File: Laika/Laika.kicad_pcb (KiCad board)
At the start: 2 copper layers, 70 x 70 mm, 29 parts, among them J1 A-DF_09_A_KG-T4S, J2 Micro_SD_Card, J3 0436500300, U1 LSM6DSL, U2 MS5611-01BA, U3 RASPBERRY_PI_ZERO_2_W, U4 MMC5983MA, U5 H3LIS331DLTR, U6 THVD1451D

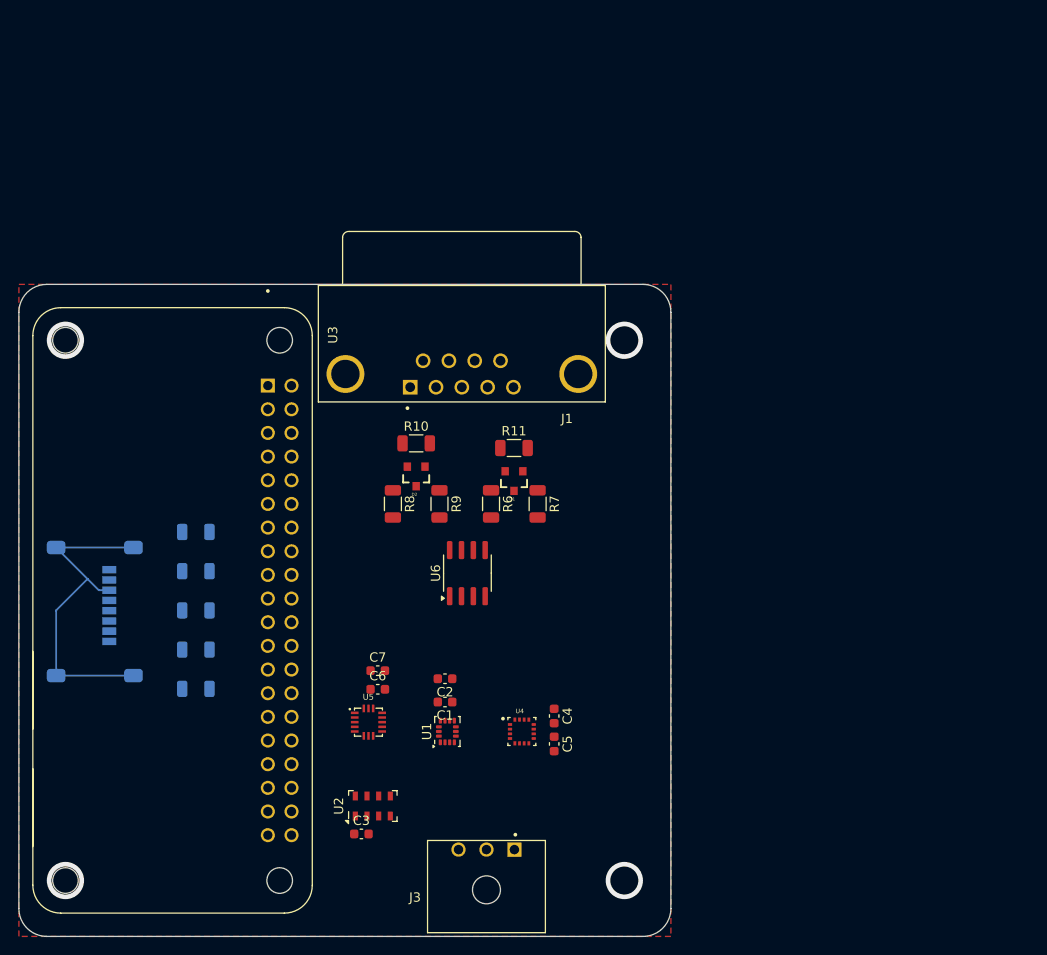
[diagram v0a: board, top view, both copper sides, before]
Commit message: Version 0A
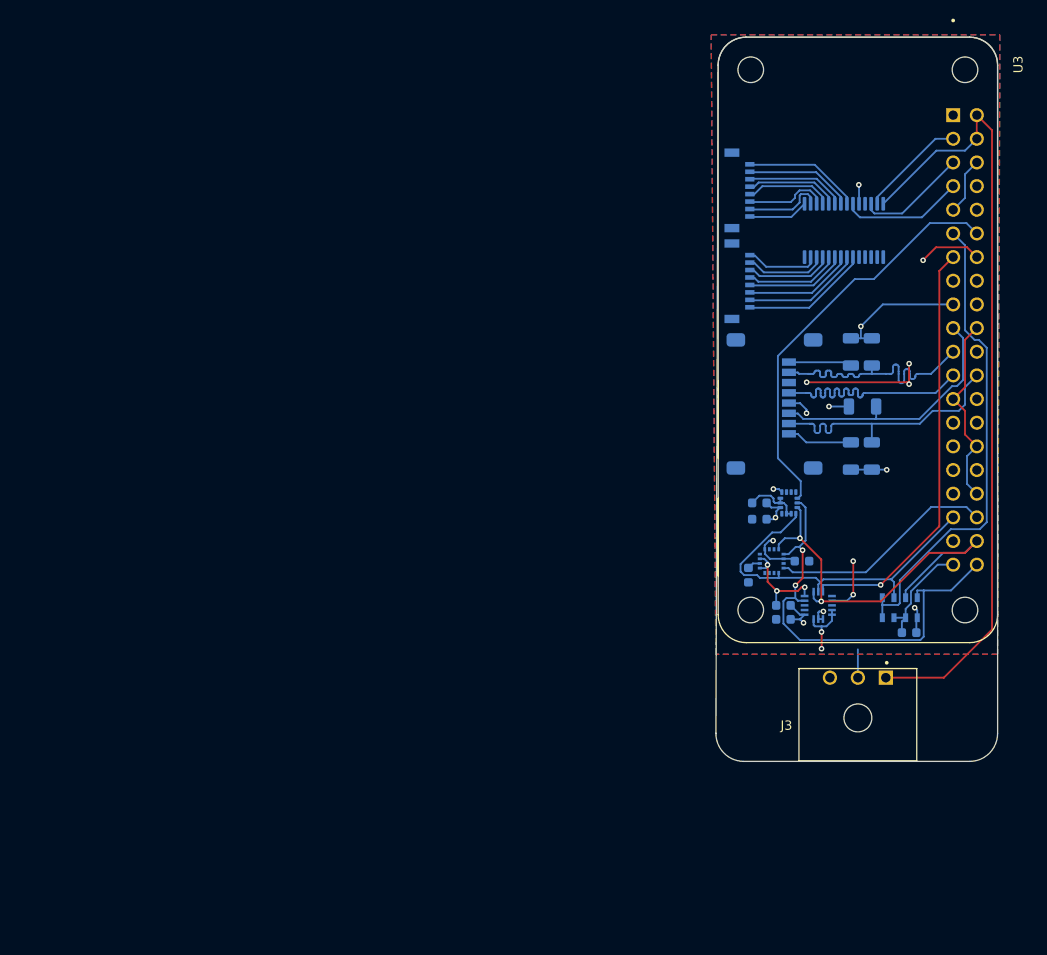
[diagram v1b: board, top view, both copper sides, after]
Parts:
- removed D1, D2: CDSOT23-SM712, CDSOT23-SM712:SOT23-3
- removed R10, R11: R, Resistor_SMD:R_1206_3216Metric
- removed R6, R7, R8, R9: 10, Resistor_SMD:R_1206_3216Metric
- added J4: DF52-8S-0.8H_21_, Hirose D52:HIROSE_DF52-8S-0.8H_21_, B.Cu at (128.5, 69.9)
- C1, C2, C3, C4, C5, C6, C7, U1, U2, U4, U5: moved to B.Cu
- J1: value A-DF_09_A_KG-T4S -> DF52-8S-0.8H_21_; footprint A-DF 09 AKG-T4S:ASSMANN_A-DF_09_A_KG-T4S -> Hirose D52:HIROSE_DF52-8S-0.8H_21_; moved to B.Cu
- U6: value THVD1451D -> PCA9685PW; footprint Package_SO:SOIC-8_3.9x4.9mm_P1.27mm -> Package_SO:TSSOP-28_4.4x9.7mm_P0.65mm; moved to B.Cu
- moved U3 79.1 mm to (140.1, 86.0)
- moved J2 76.3 mm to (130.6, 92.8)
- moved R2 76.3 mm to (141.6, 87.2), turned to -90 degrees
- moved R4 75.5 mm to (141.6, 98.4), turned to 90 degrees
- moved R3 74.8 mm to (140.6, 93.1), turned to 0 degrees
- moved R5 74.6 mm to (139.3, 98.4), turned to 90 degrees
- moved R1 72.9 mm to (139.3, 87.2), turned to -90 degrees
- moved C3 62.6 mm to (145.6, 117.4), turned to 180 degrees
- moved U2 60.4 mm to (144.6, 114.7)
- moved U6 54.7 mm to (138.6, 74.2)
- moved U5 49.9 mm to (135.8, 114.5)
- moved C6 44.5 mm to (132.1, 114.5), turned to 180 degrees
- moved U1 44.1 mm to (132.7, 103.5)
- moved J3 43.9 mm to (140.1, 122.2)
- moved C7 43.9 mm to (132.1, 116.0), turned to 180 degrees
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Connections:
- J1 pad 1: unconnected-(J1-Pad1) -> PWM_0
- J1 pad 2: MODBUS_RX_P -> PWM_1
- J1 pad 3: MODBUS_TX_P -> PWM_2
- J1 pad 4: unconnected-(J1-Pad4) -> PWM_3
- J1 pad 5: GND -> PWM_4
- J1 pad 6: unconnected-(J1-Pad6) -> PWM_5
- J1 pad 7: unconnected-(J1-Pad7) -> PWM_6
- J1 pad 8: MODBUS_RX_N -> PWM_7
- U6 pad 1: +3.3V -> GND
- U6 pad 2: PI_UART_RX -> GND
- U6 pad 3: PI_UART_TX -> GND
- U6 pad 5: Net-(U6-Y) -> GND
- U6 pad 6: Net-(U6-Z) -> PWM_0
- U6 pad 7: Net-(U6-B) -> PWM_1
- U6 pad 8: Net-(U6-A) -> PWM_2
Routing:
- net +5V: track 0.00 -> 84.9 mm
- net GND: track 36.0 -> 94.2 mm, vias 0 -> 12
- net BUS_SPI1_CE1: track 0.00 -> 51.3 mm
- net BUS_SPI1_SCLK: track 0.00 -> 47.7 mm, vias 0 -> 2
- net BUS_SPI1_MOSI: track 0.00 -> 46.0 mm, vias 0 -> 2
- net PI_GPIO_27: track 0.00 -> 45.3 mm, vias 0 -> 1
- net BUS_SPI1_CE0: track 0.00 -> 44.2 mm
- net +3.3V: track 0.00 -> 42.5 mm, vias 0 -> 10
- net BUS_SPI1_MISO: track 0.00 -> 39.3 mm
- net BUS_SPI0_MOSI: track 0.00 -> 28.8 mm
- net BUS_SPI0_CE0: track 0.00 -> 28.6 mm
- net BUS_SPI0_MISO: track 0.00 -> 27.4 mm
- net BUS_SPI0_SCLK: track 0.00 -> 26.2 mm
- net BUS_SPI1_CE2: track 0.00 -> 24.3 mm
- net PWM_0: track 0.00 -> 14.0 mm
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- added copper zone on F.Cu, net +3.3V
- added copper zone on B.Cu, net GND
- removed copper zone on F.Cu, net GND
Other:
- board size 70 x 70 mm -> 30.2 x 77.8 mm
- board text added: "Laika Flight Computer"
- board text added: "Made on Earth by Humans"
- board text added: "Rev 0A"
